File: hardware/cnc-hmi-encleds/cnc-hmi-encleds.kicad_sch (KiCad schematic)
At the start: 48 parts, among them J1 Conn_01x04, U1 SN74LVC1T45DBV

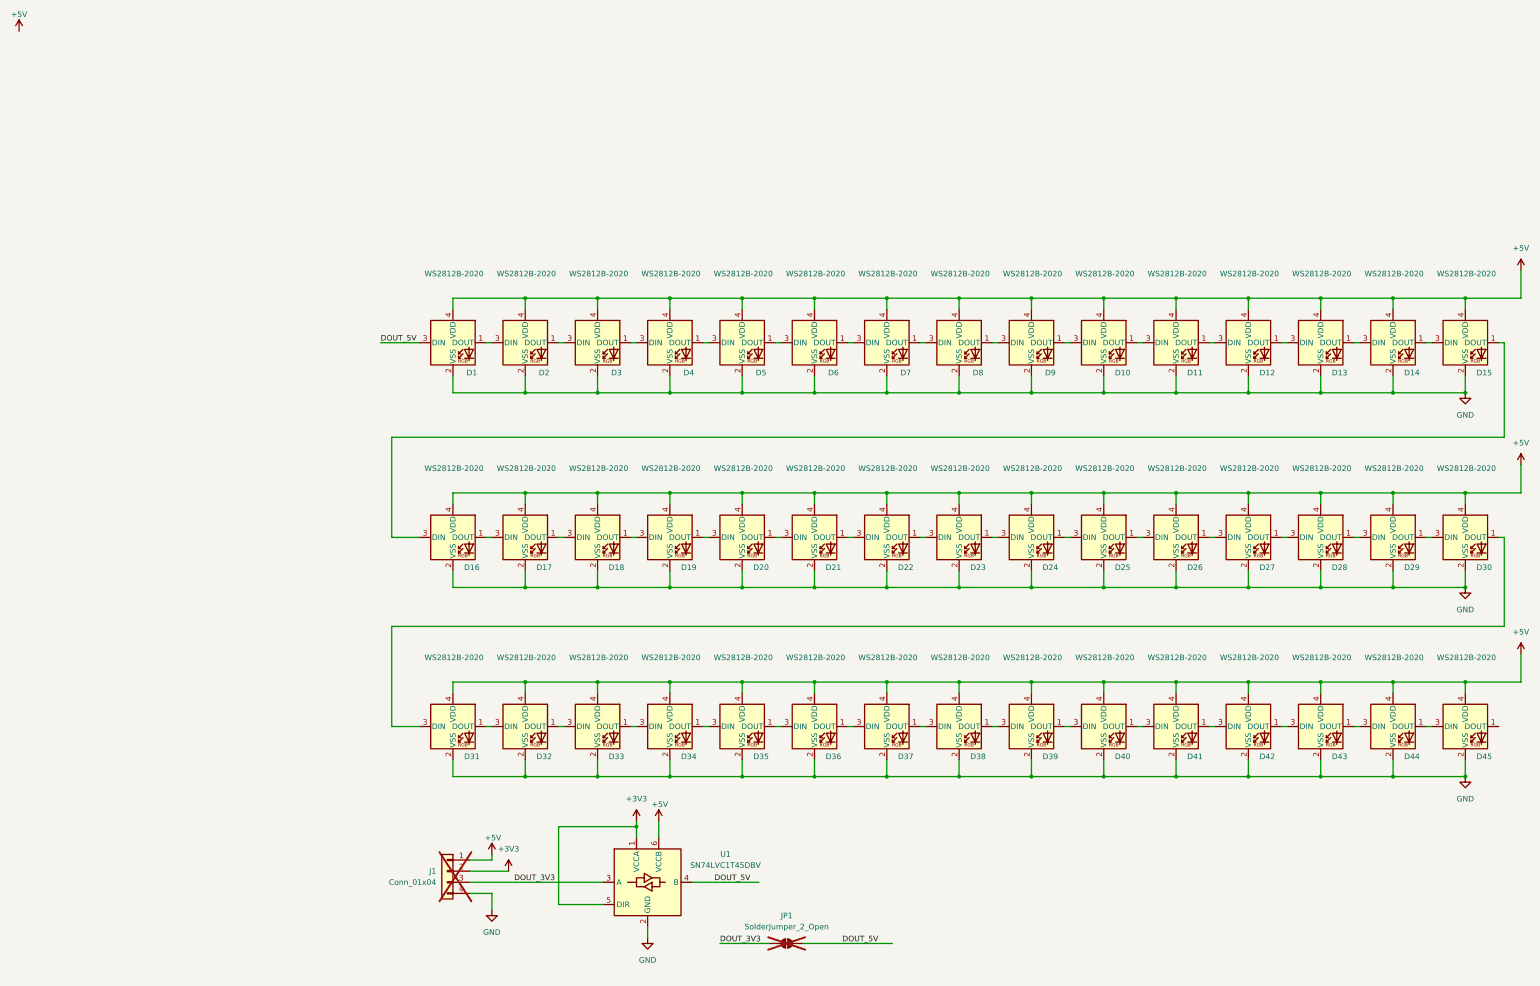
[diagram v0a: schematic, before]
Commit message: prep for fab&assembly
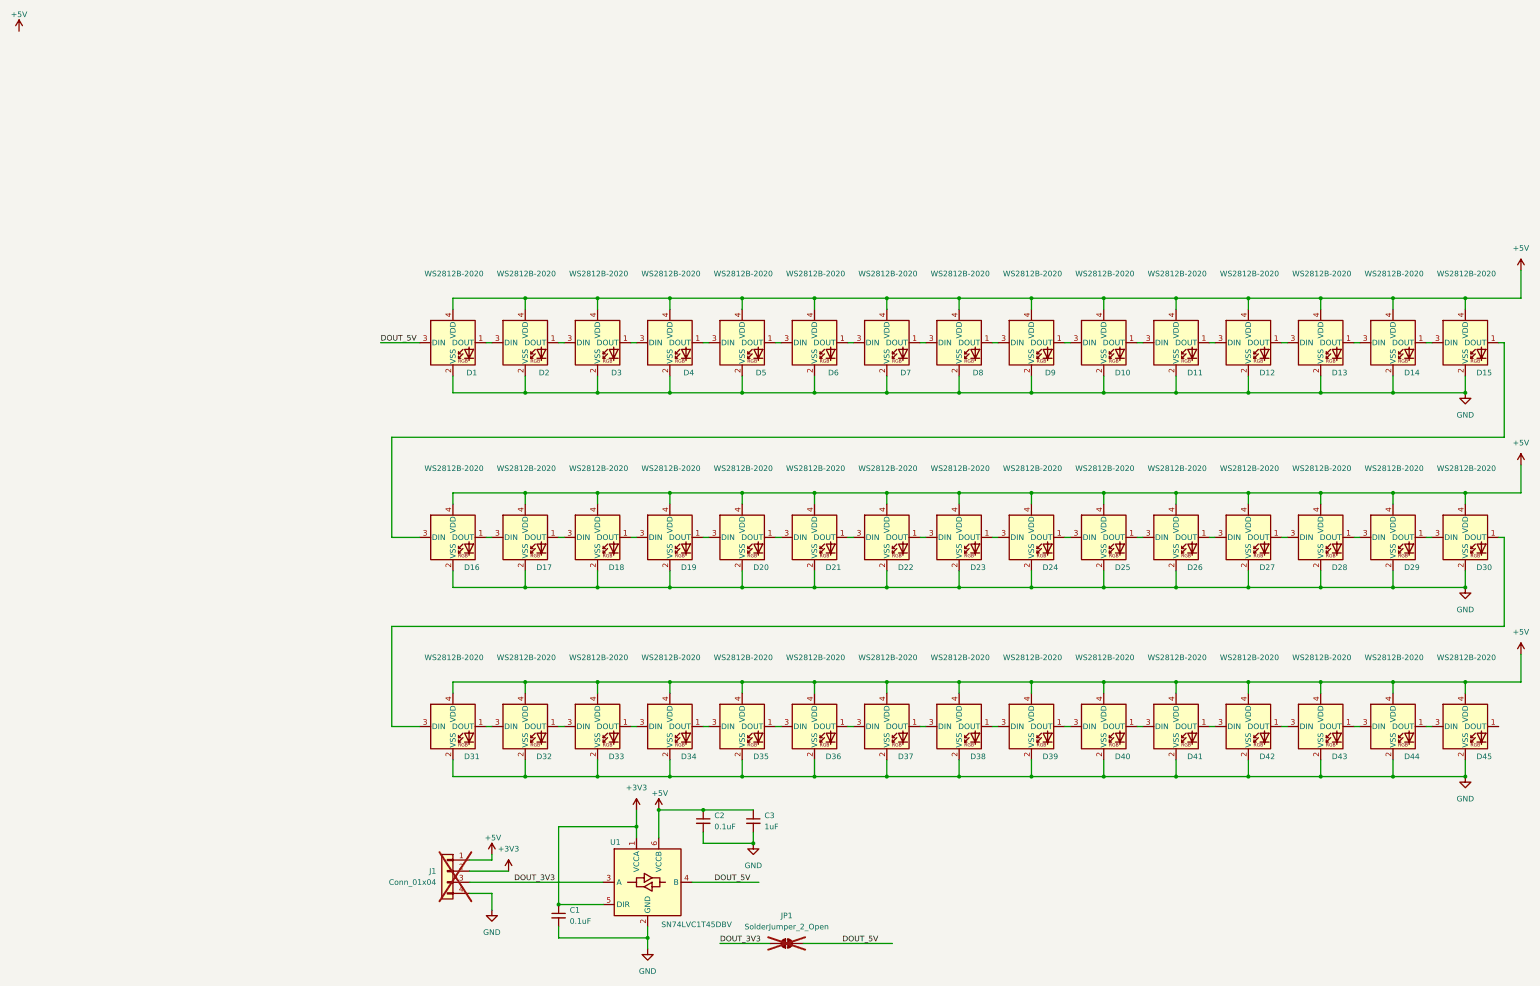
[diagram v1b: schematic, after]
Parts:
- added C1, C2: 0.1uF, Capacitor_SMD:C_0603_1608Metric, symbol Device:C_Small
- added C3: 1uF, Capacitor_SMD:C_0805_2012Metric, symbol Device:C_Small
- D1, D10, D11, D12, D13, D14, D15, D16, D17, D18, D19, D2, D20, D21, D22, D23, D24, D25, D26, D27, D28, D29, D3, D30, D31, D32, D33, D34, D35, D36, D37, D38, D39, D4, D40, D41, D42, D43, D44, D45, D5, D6, D7, D8, D9: footprint EncLEDS Library:LED_WS2812B-2020_PLCC4_2.0x2.0mm -> LED_SMD:LED_WS2812B-2020_PLCC4_2.0x2.0mm; symbol LED:WS2812B-2020 -> EncLEDS Library:WS2812B-2020; JLCPCB P/N (none) -> C965555
- U1: JLCPCB P/N (none) -> C7843
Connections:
- net +3V3: now also C1.1
- net +5V: now also C2.1, C3.1
- net GND: now also C1.2, C2.2, C3.2
